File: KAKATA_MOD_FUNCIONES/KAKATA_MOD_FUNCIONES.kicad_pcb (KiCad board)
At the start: 4 copper layers, 57.7 x 42.6 mm, 30 parts, among them CN1 HX JN1.27-2X3 TP H4.9, U1 ESP32-S3-WROOM-1(N16R8), U10 DB125-2.54-4P-GN, U11 DB125-2.54-4P-GN, U12 DB125-2.54-4P-GN, U13 DB125-2.54-4P-GN, U14 DB125-2.54-4P-GN, U2 PSC-1608U52GC-G4, U3 PSC-1608U52GC-G4, U4 PSC-1608U52GC-G4, U5 PSC-1608U52GC-G4, U6 SMQP-02R-TP, U7 DB125-3.5-2P-GN-S, U8 DB125-3.5-2P-GN-S

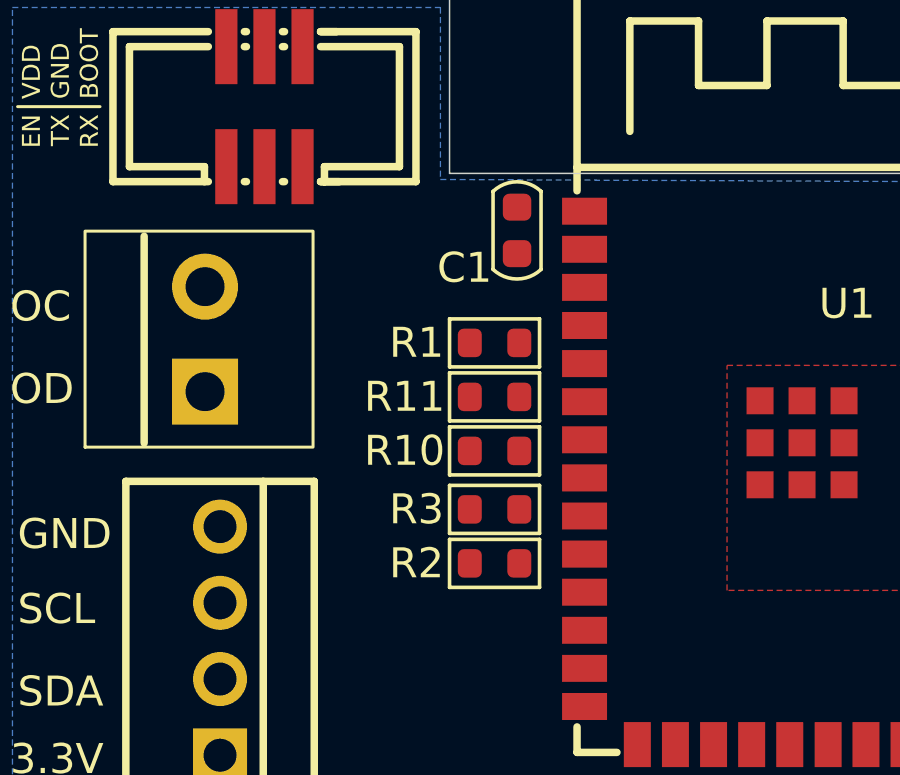
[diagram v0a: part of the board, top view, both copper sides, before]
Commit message: hot_fix_Done
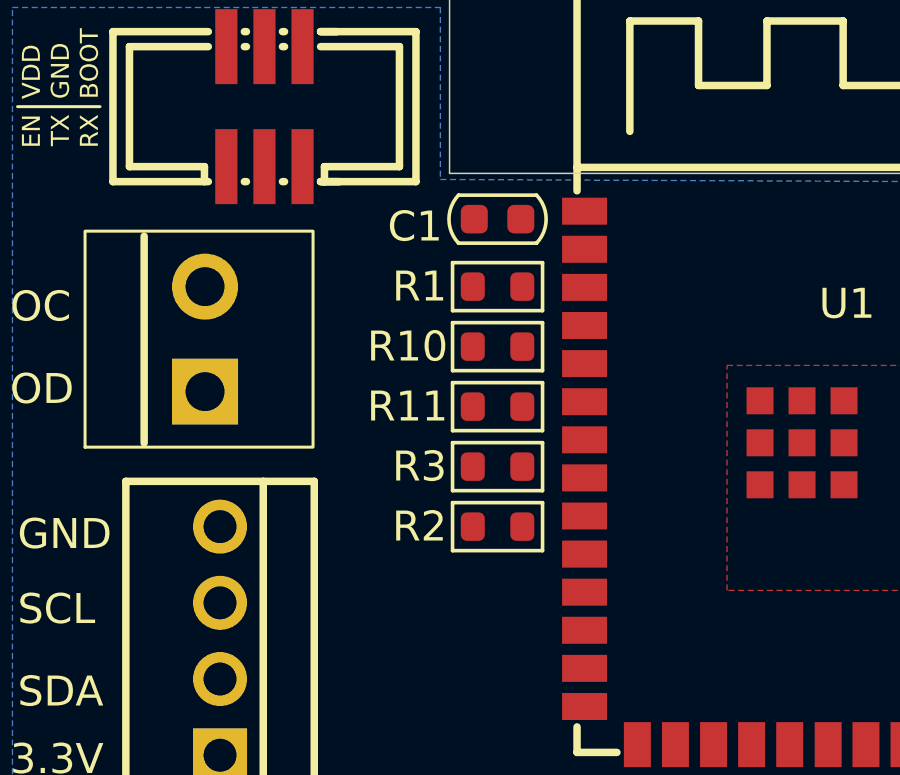
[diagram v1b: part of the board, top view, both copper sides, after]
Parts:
- moved R10 3.48 mm to (96.6, 45.0)
- moved R1 1.88 mm to (96.6, 43.0)
- moved R3 1.43 mm to (96.6, 49.0)
- moved R2 1.23 mm to (96.6, 51.0)
- moved C1 0.75 mm to (96.6, 40.8), turned to 0 degrees
- moved R11 0.34 mm to (96.6, 47.0)
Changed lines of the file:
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@@
 	(footprint "PCM_Resistor_SMD_AKL:R_0603_1608Metric"
 		(layer "F.Cu")
-		(at 96.5 46.7 180)
+		(at 96.6 47.025 180)
 		(descr "Resistor SMD 0603 (1608 Metric), square (rectangular) end terminal, IPC_7351 nominal, (Body size source: IPC-SM-782 page 72, https://www.pcb-3d.com/wordpress/wp-content/uploads/ipc-sm-782a_amendment_1_and_2.pdf), Alternate KiCad Library")
 		(tags "resistor")
@@
 	(footprint "PCM_Resistor_SMD_AKL:R_0603_1608Metric"
 		(layer "F.Cu")
-		(at 96.5 48.5 180)
+		(at 96.6 45.025 180)
 		(descr "Resistor SMD 0603 (1608 Metric), square (rectangular) end terminal, IPC_7351 nominal, (Body size source: IPC-SM-782 page 72, https://www.pcb-3d.com/wordpress/wp-content/uploads/ipc-sm-782a_amendment_1_and_2.pdf), Alternate KiCad Library")
 		(tags "resistor")
@@
 	(footprint "PCM_Resistor_SMD_AKL:R_0603_1608Metric"
 		(layer "F.Cu")
-		(at 96.5 52.25)
+		(at 96.6 51.025)
 		(descr "Resistor SMD 0603 (1608 Metric), square (rectangular) end terminal, IPC_7351 nominal, (Body size source: IPC-SM-782 page 72, https://www.pcb-3d.com/wordpress/wp-content/uploads/ipc-sm-782a_amendment_1_and_2.pdf), Alternate KiCad Library")
 		(tags "resistor")
@@
 	(footprint "PCM_Resistor_SMD_AKL:R_0603_1608Metric"
 		(layer "F.Cu")
-		(at 96.5 50.45)
+		(at 96.6 49.025)
 		(descr "Resistor SMD 0603 (1608 Metric), square (rectangular) end terminal, IPC_7351 nominal, (Body size source: IPC-SM-782 page 72, https://www.pcb-3d.com/wordpress/wp-content/uploads/ipc-sm-782a_amendment_1_and_2.pdf), Alternate KiCad Library")
 		(tags "resistor")
@@
 	(footprint "PCM_Resistor_SMD_AKL:R_0603_1608Metric"
 		(layer "F.Cu")
-		(at 96.5 44.9)
+		(at 96.6 43.025)
 		(descr "Resistor SMD 0603 (1608 Metric), square (rectangular) end terminal, IPC_7351 nominal, (Body size source: IPC-SM-782 page 72, https://www.pcb-3d.com/wordpress/wp-content/uploads/ipc-sm-782a_amendment_1_and_2.pdf), Alternate KiCad Library")
 		(tags "resistor")
@@
 	(footprint "PCM_Capacitor_SMD_AKL:C_0603_1608Metric"
 		(layer "F.Cu")
-		(at 97.25 41.15 -90)
+		(at 96.6 40.775)
 		(descr "Capacitor SMD 0603 (1608 Metric), square (rectangular) end terminal, IPC_7351 nominal, (Body size source: IPC-SM-782 page 76, https://www.pcb-3d.com/wordpress/wp-content/uploads/ipc-sm-782a_amendment_1_and_2.pdf), Alternate KiCad Library")
 		(tags "capacitor")
 		(property "Reference" "C1"
-			(at 1.25 1.75 0)
+			(at -2.75 0.25 180)
 			(layer "F.SilkS")
 			(effects
@@
 		)
 		(property "Value" "C_0603"
-			(at 0 1.43 90)
+			(at 0 1.43 0)
 			(layer "F.Fab")
 			(hide yes)
@@
 		)
 		(property "Datasheet" "~"
-			(at 0 0 90)
+			(at 0 0 0)
 			(layer "F.Fab")
 			(hide yes)
@@
 		)
 		(property "Description" "SMD 0603 MLCC capacitor, Alternate KiCad Library"
-			(at 0 0 90)
+			(at 0 0 0)
 			(layer "F.Fab")
 			(hide yes)
@@
 		)
 		(fp_line
-			(start -1.48 0.73)
-			(end -1.48 -0.73)
+			(start -1.48 -0.73)
+			(end 1.48 -0.73)
 			(stroke
 				(width 0.05)
@@
 		)
 		(fp_line
-			(start 1.48 0.73)
-			(end -1.48 0.73)
+			(start -1.48 0.73)
+			(end -1.48 -0.73)
 			(stroke
 				(width 0.05)
@@
 		)
 		(fp_line
-			(start -1.48 -0.73)
-			(end 1.48 -0.73)
+			(start 1.48 -0.73)
+			(end 1.48 0.73)
 			(stroke
 				(width 0.05)
@@
 		)
 		(fp_line
-			(start 1.48 -0.73)
-			(end 1.48 0.73)
+			(start 1.48 0.73)
+			(end -1.48 0.73)
 			(stroke
 				(width 0.05)
@@
 		)
 		(fp_line
-			(start -0.8 0.4)
-			(end -0.8 -0.4)
+			(start -0.8 -0.4)
+			(end 0.8 -0.4)
 			(stroke
 				(width 0.1)
@@
 		)
 		(fp_line
-			(start 0.8 0.4)
-			(end -0.8 0.4)
+			(start -0.8 0.4)
+			(end -0.8 -0.4)
 			(stroke
 				(width 0.1)
@@
 		)
 		(fp_line
-			(start -0.8 -0.4)
-			(end 0.8 -0.4)
+			(start 0.8 -0.4)
+			(end 0.8 0.4)
 			(stroke
 				(width 0.1)
@@
 		)
 		(fp_line
-			(start 0.8 -0.4)
-			(end 0.8 0.4)
+			(start 0.8 0.4)
+			(end -0.8 0.4)
 			(stroke
 				(width 0.1)
@@
 		)
 		(fp_text user "${REFERENCE}"
-			(at 0.8 0 90)
+			(at 0.8 0 0)
 			(layer "F.Fab")
 			(effects
@@
 		)
 		(pad "1" smd roundrect
-			(at -0.775 0 270)
+			(at -0.775 0)
 			(size 0.9 0.95)
 			(layers "F.Cu" "F.Mask" "F.Paste")
@@
 		)
 		(pad "2" smd roundrect
-			(at 0.775 0 270)
+			(at 0.775 0)
 			(size 0.9 0.95)
 			(layers "F.Cu" "F.Mask" "F.Paste")
